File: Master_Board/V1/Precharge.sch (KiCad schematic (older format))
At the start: 24 parts, among them J701 649002227222, J702 649002227222, Q701 BC849BLT1G, Q702 BC849BLT1G, U701 LTV-816S, U702 LTV-816S

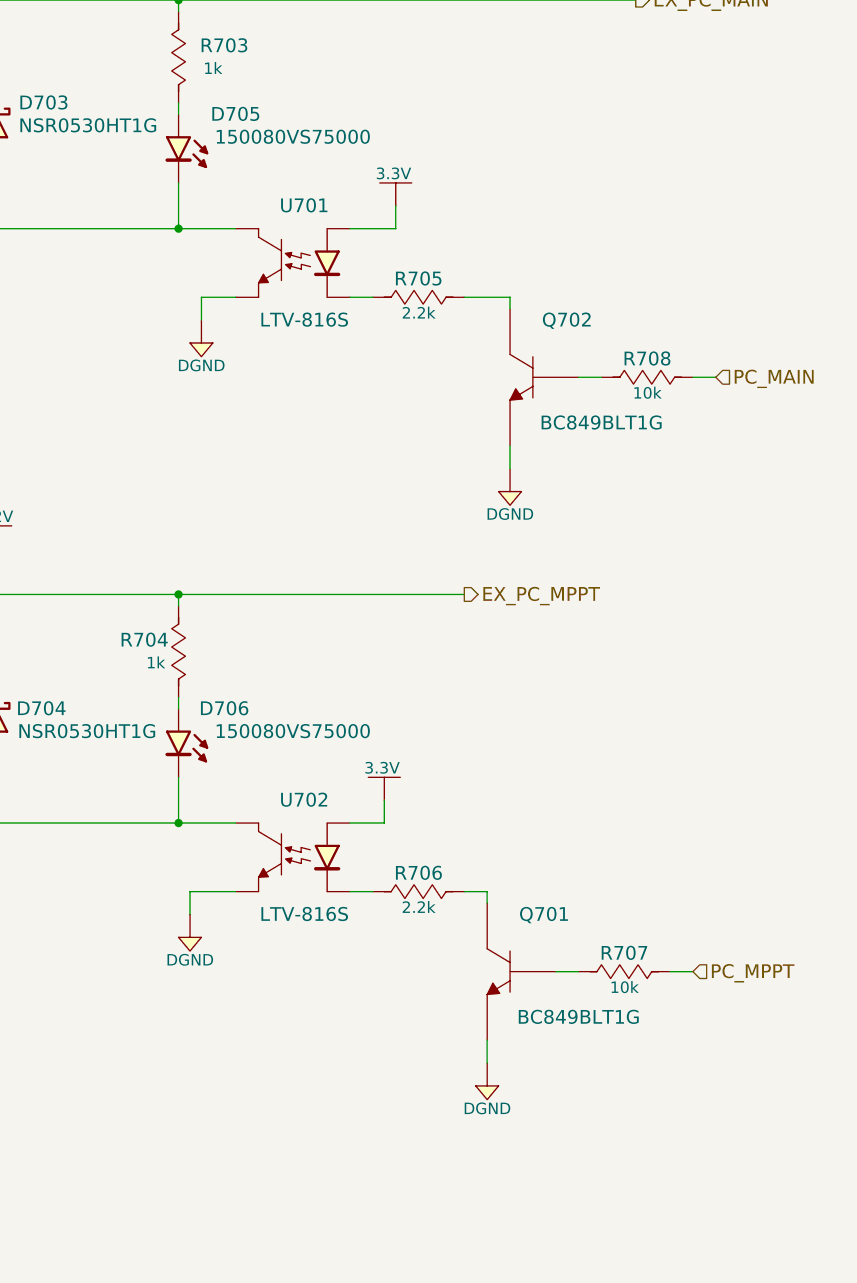
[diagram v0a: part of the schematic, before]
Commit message: Routing BmsMasterBoard
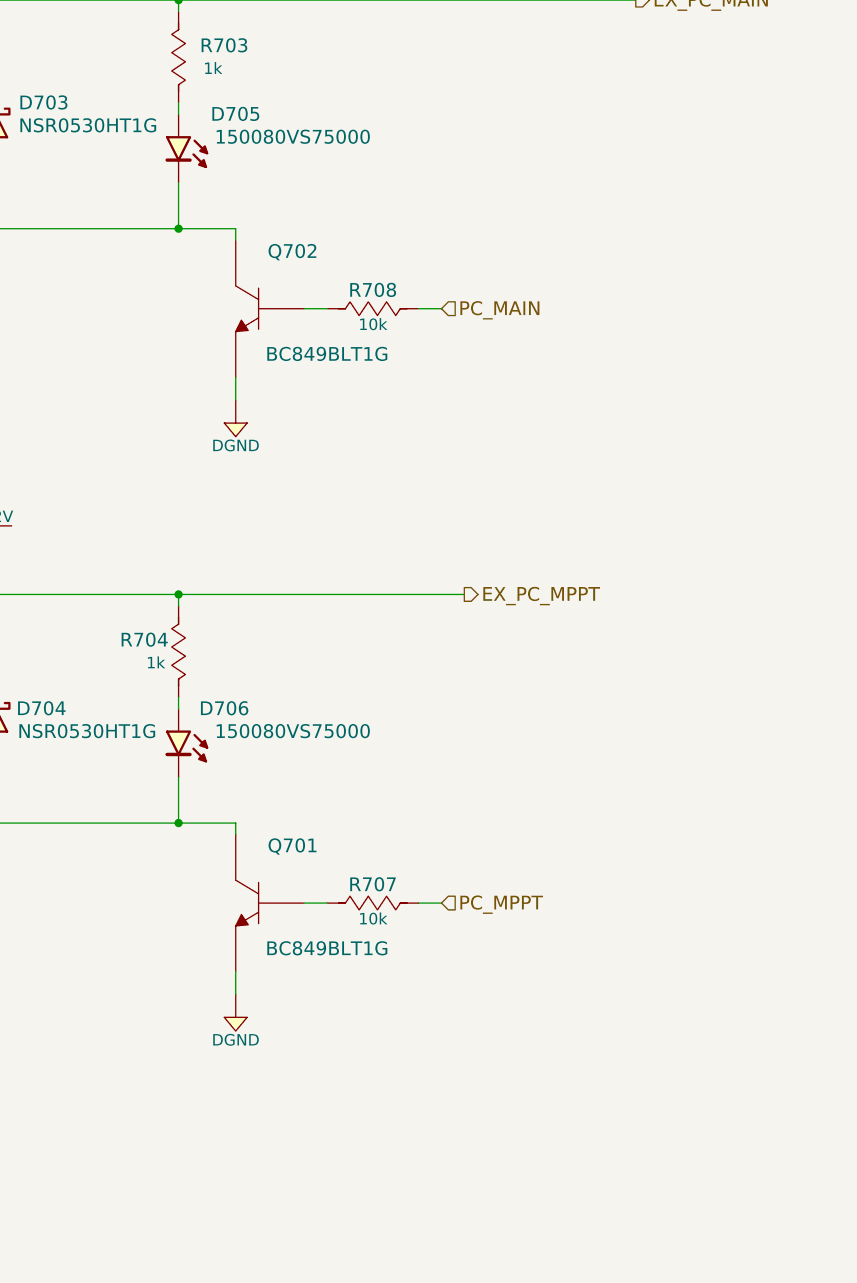
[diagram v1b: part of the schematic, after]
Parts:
- removed R705, R706: RC0805JR-072K2L, Resistors:R0805, symbol RC0805JR-072K2L
- removed U701, U702: LTV-816S, IC:4-SMD, symbol LTV-816S-RESCUE-Master_Board
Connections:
- net at D703.2 (Anode), D705.1 (Cathode), RL702.1: now also Q702.3 (C)
- net at D704.2 (Anode), D706.1 (Cathode), RL701.1: now also Q701.3 (C)
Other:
- moved on the sheet: Q701, Q702, R707, R708
